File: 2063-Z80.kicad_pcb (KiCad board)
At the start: 4 copper layers, 100 x 100 mm, 87 parts, among them J1 Conn_01x05, J10 Conn_01x07, J11 Conn_02x03, J12 Conn_01x02, J2 DM3D-SF(41), J3 Conn_02x20, J3A1 Conn_02x02_Odd_Even, J4 Conn_02x05, J5 Conn_02x05, J6 0548190519, J7 Conn_02x13, J8 Conn_01x05, J9 Conn_01x02, Q1 PN2222, U1 Z80-CPU, U10 74HC32, U11 74HCT132, U12 ICL3232CPZ, U13 74HC32, U2 AS6C4008-55PCN, U20 LM1117-3.3, U3 SST39SF010, U4 Z80-CTC, U5 Z80-SIO-0, U6 74HC374, U7 74HC374, U8 74LS244, U9 74HC138, X1 ACH-10.000MHZ-EK, X2 ECS-2100A-018

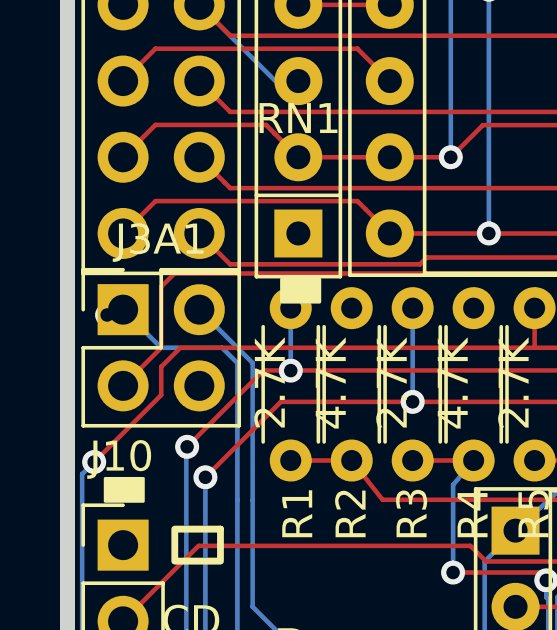
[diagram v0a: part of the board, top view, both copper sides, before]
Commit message: Modified to fit my needs.
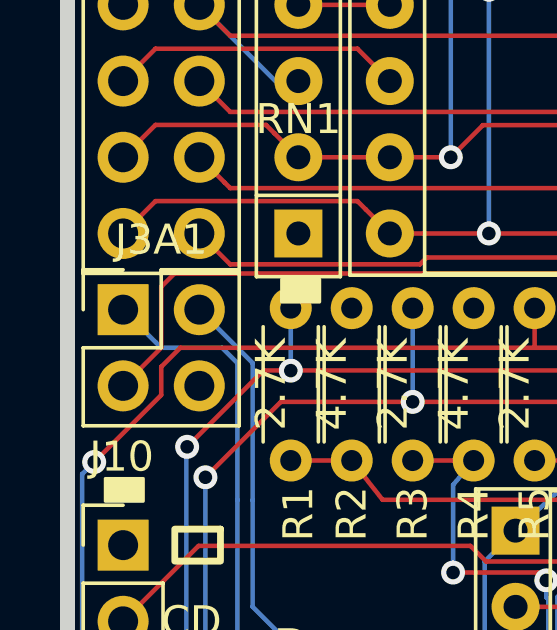
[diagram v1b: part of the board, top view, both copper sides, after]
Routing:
- net /~IORQ_50: vias 3 -> 2
